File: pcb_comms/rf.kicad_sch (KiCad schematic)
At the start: 25 parts, among them J4 Conn_Coaxial, U2 CG2179M2

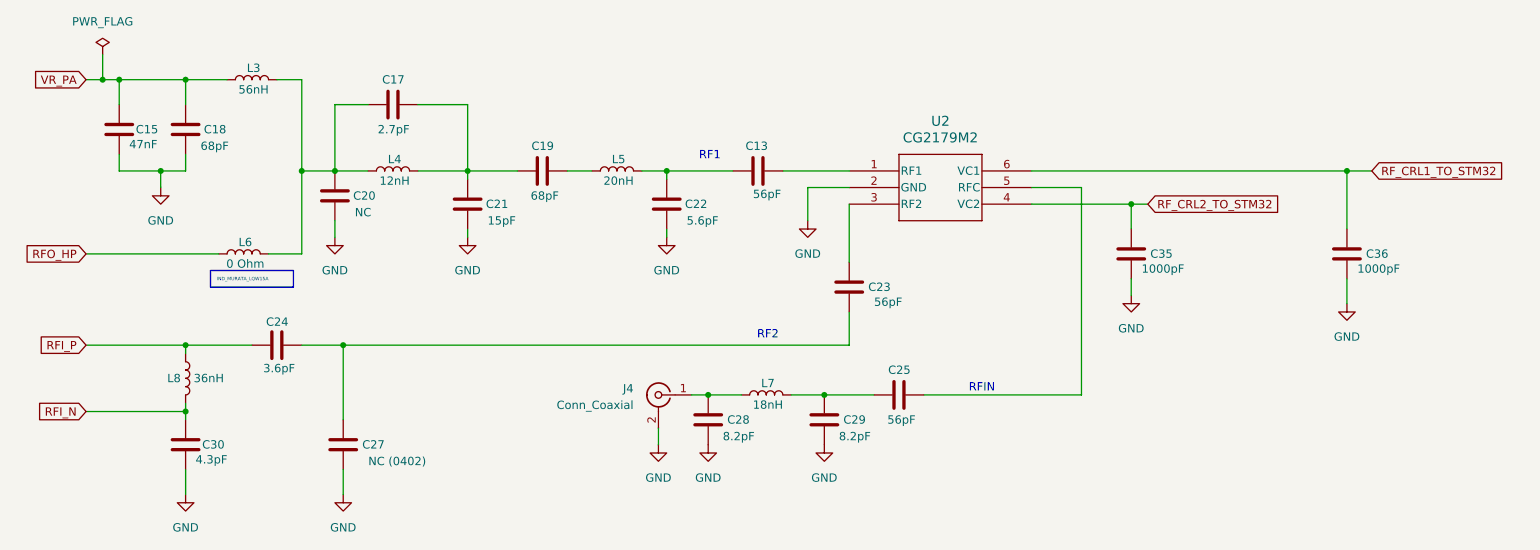
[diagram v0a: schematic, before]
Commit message: Last update
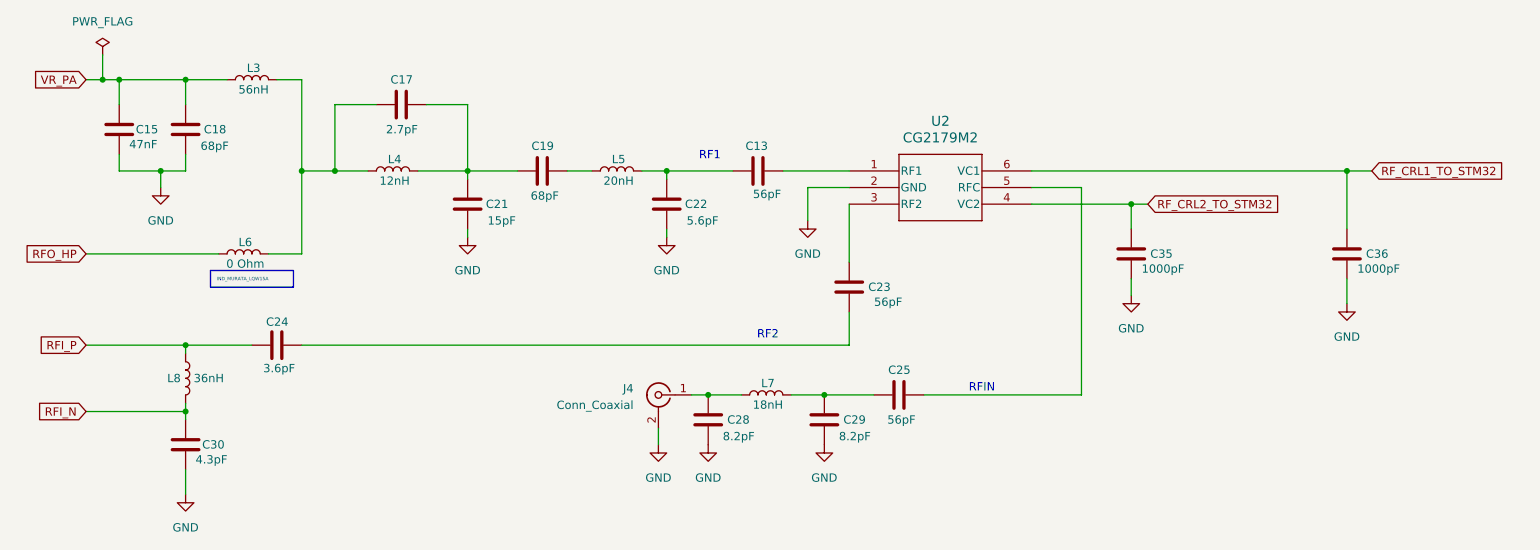
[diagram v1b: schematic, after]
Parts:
- removed C20: NC, symbol Device:C
- removed C27: NC (0402), symbol Device:C
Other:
- company: (none) -> Sanie Peralta, Alejandro Campo
- title: (none) -> PC1: APRS & GPS
- moved on the sheet: C17
